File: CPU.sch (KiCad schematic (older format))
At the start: 20 parts, among them J301 Molex+Microfit3-Dual4-90, J302 Conn_02x18_Odd_Even, U301 MC9S12XEP100, Y301 16mHz

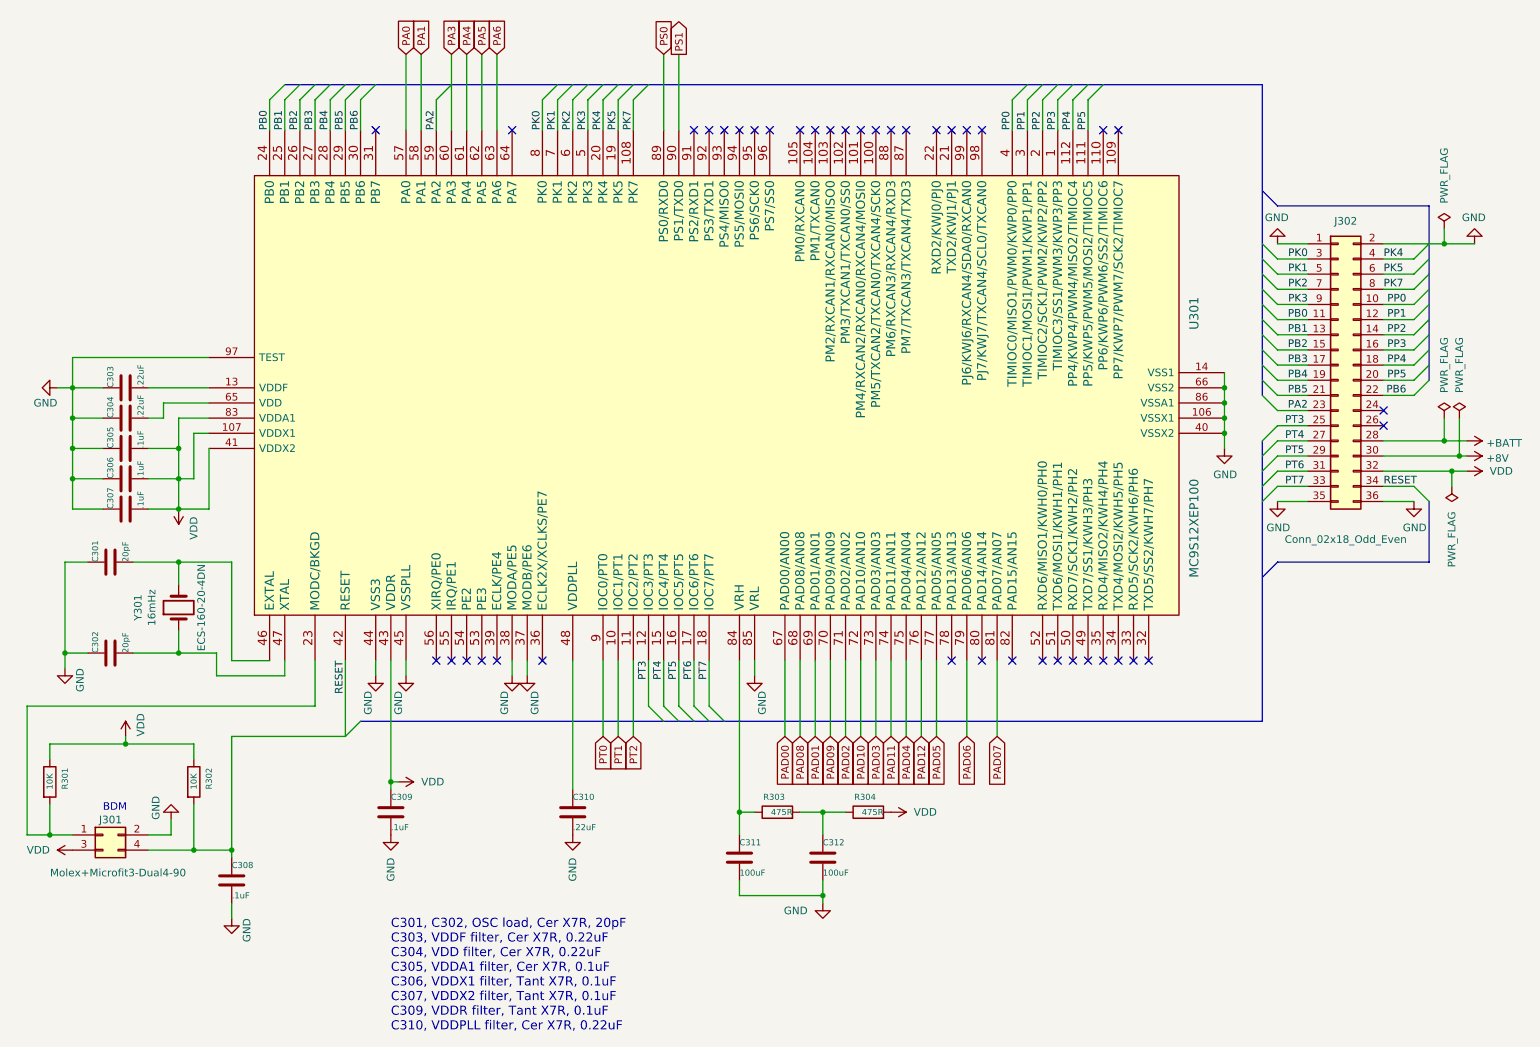
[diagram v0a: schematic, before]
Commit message: Add files via upload
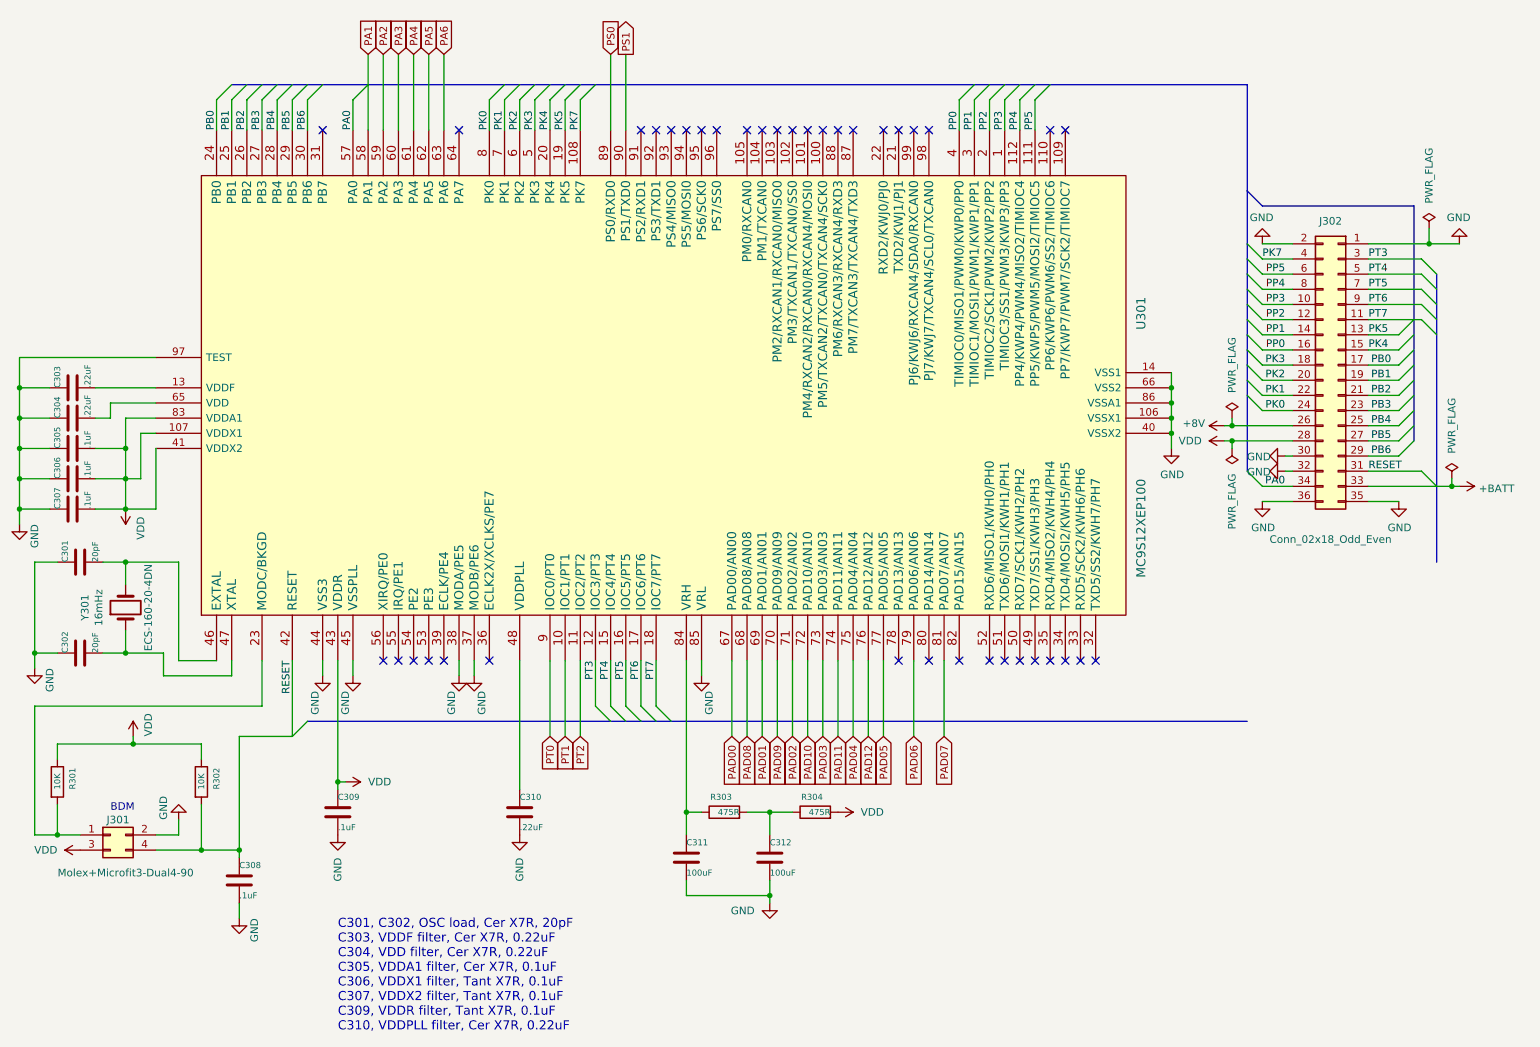
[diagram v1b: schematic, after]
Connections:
- net +8V: now also J302.26 (Pin_26); no longer J302.30 (Pin_30)
- net +BATT: now also J302.33 (Pin_33); no longer J302.28 (Pin_28)
- net GND: now also J302.30 (Pin_30), J302.32 (Pin_32)
- net PA0: now also J302.34 (Pin_34)
- net PA2: no longer J302.23 (Pin_23)
- net PB0: now also J302.17 (Pin_17); no longer J302.11 (Pin_11)
- net PB1: now also J302.19 (Pin_19); no longer J302.13 (Pin_13)
- net PB2: now also J302.21 (Pin_21); no longer J302.15 (Pin_15)
- net PB3: now also J302.23 (Pin_23); no longer J302.17 (Pin_17)
- net PB4: now also J302.25 (Pin_25); no longer J302.19 (Pin_19)
- net PB5: now also J302.27 (Pin_27); no longer J302.21 (Pin_21)
- net PB6: now also J302.29 (Pin_29); no longer J302.22 (Pin_22)
- net PK0: now also J302.24 (Pin_24); no longer J302.3 (Pin_3)
- net PK1: now also J302.22 (Pin_22); no longer J302.5 (Pin_5)
- net PK2: now also J302.20 (Pin_20); no longer J302.7 (Pin_7)
- net PK3: now also J302.18 (Pin_18); no longer J302.9 (Pin_9)
- net PK4: now also J302.15 (Pin_15); no longer J302.4 (Pin_4)
- net PK5: now also J302.13 (Pin_13); no longer J302.6 (Pin_6)
- net PK7: now also J302.4 (Pin_4); no longer J302.8 (Pin_8)
- net PP0: now also J302.16 (Pin_16); no longer J302.10 (Pin_10)
- net PP1: now also J302.14 (Pin_14); no longer J302.12 (Pin_12)
- net PP2: now also J302.12 (Pin_12); no longer J302.14 (Pin_14)
- net PP3: now also J302.10 (Pin_10); no longer J302.16 (Pin_16)
- net PP4: now also J302.8 (Pin_8); no longer J302.18 (Pin_18)
- net PP5: now also J302.6 (Pin_6); no longer J302.20 (Pin_20)
- net PT3: now also J302.3 (Pin_3); no longer J302.25 (Pin_25)
- net PT4: now also J302.5 (Pin_5); no longer J302.27 (Pin_27)
- net PT5: now also J302.7 (Pin_7); no longer J302.29 (Pin_29)
- net PT6: now also J302.9 (Pin_9); no longer J302.31 (Pin_31)
- net PT7: now also J302.11 (Pin_11); no longer J302.33 (Pin_33)
- net RESET: now also J302.31 (Pin_31); no longer J302.34 (Pin_34)
- net VDD: now also J302.28 (Pin_28); no longer J302.32 (Pin_32)
- no-connect marks 41 -> 39
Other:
- moved on the sheet: C301, C302, C303, C304, C305, C306, C307, C308, C309, C310, C311, C312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
